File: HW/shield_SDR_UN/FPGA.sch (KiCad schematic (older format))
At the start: 68 parts, among them J1 Conn_02x09_Odd_Even, J2 Conn_02x08_Odd_Even, U4 XC6SLX9-2TQG144C, X2 ASE-xxxMHz

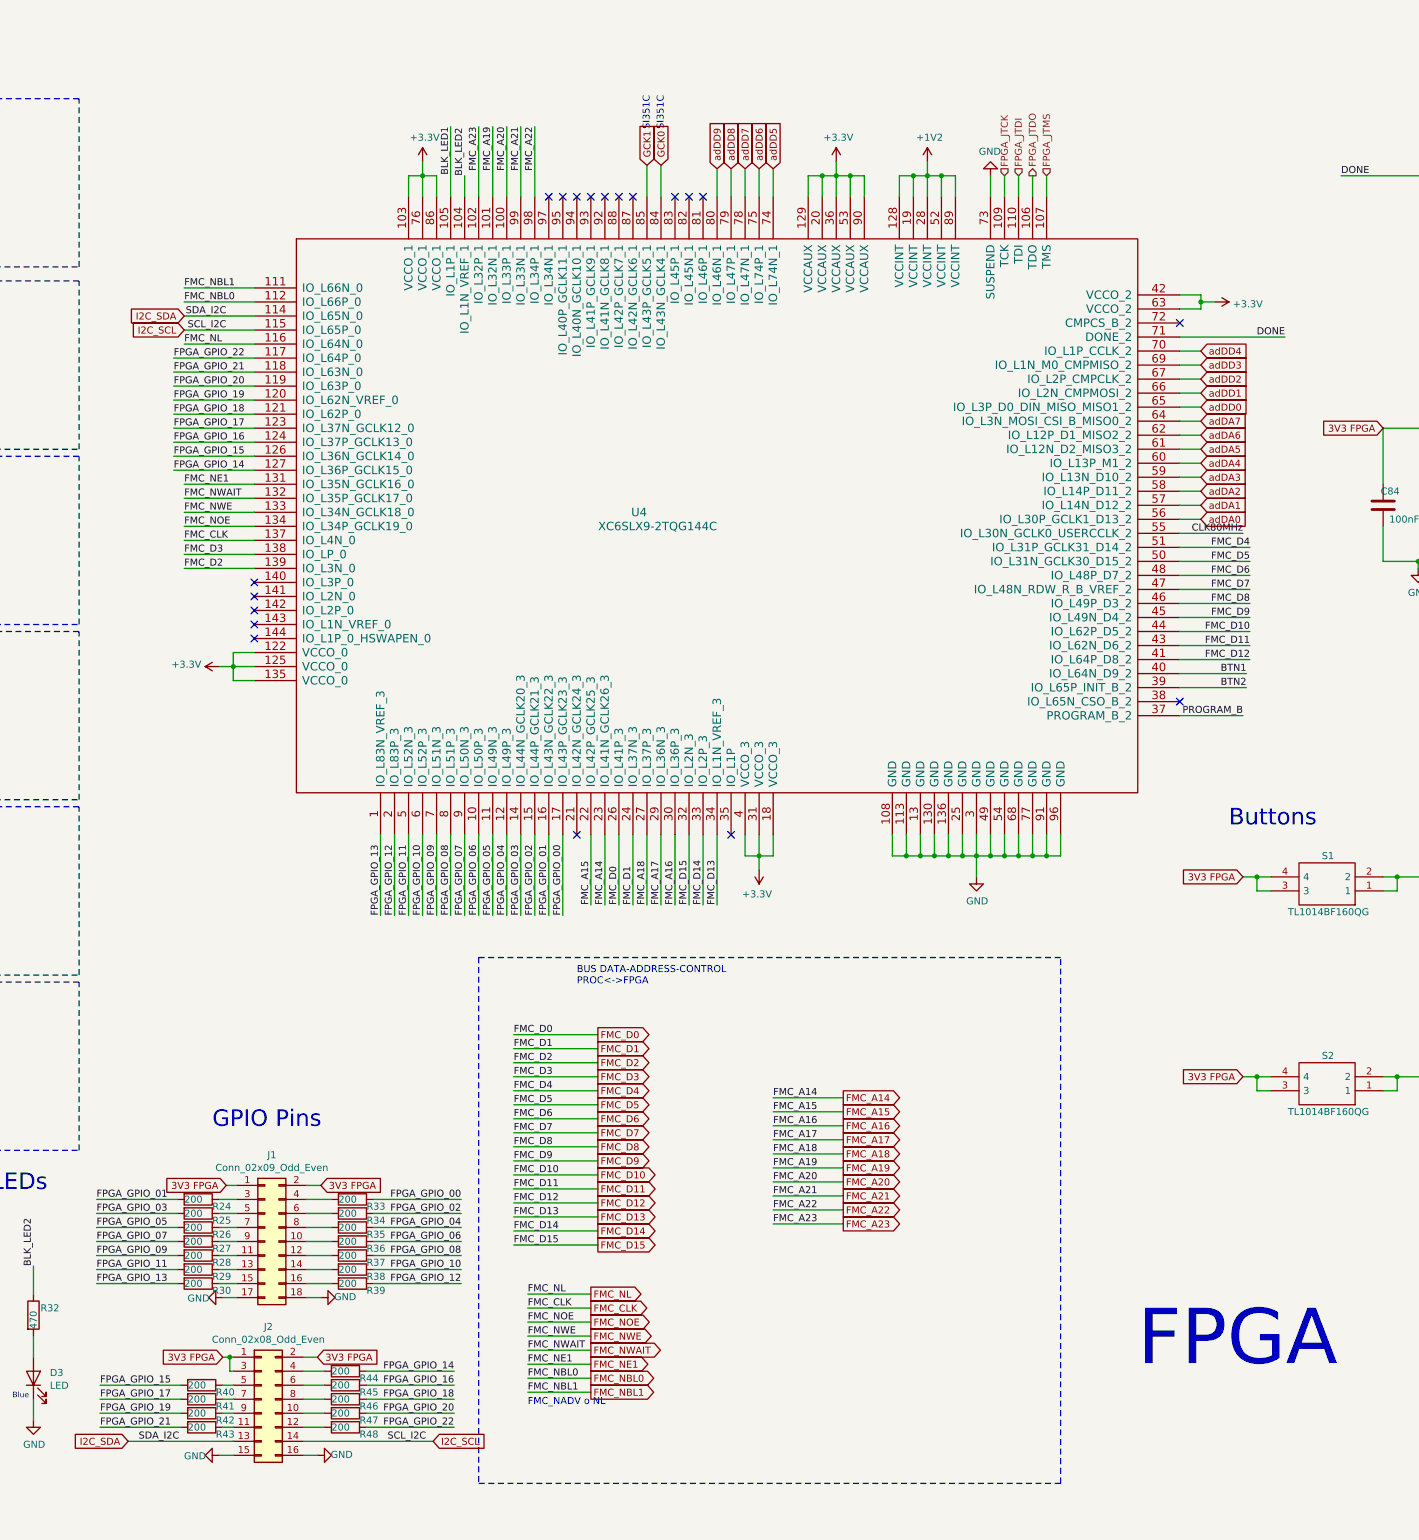
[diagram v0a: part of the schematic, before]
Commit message: PCB route V3
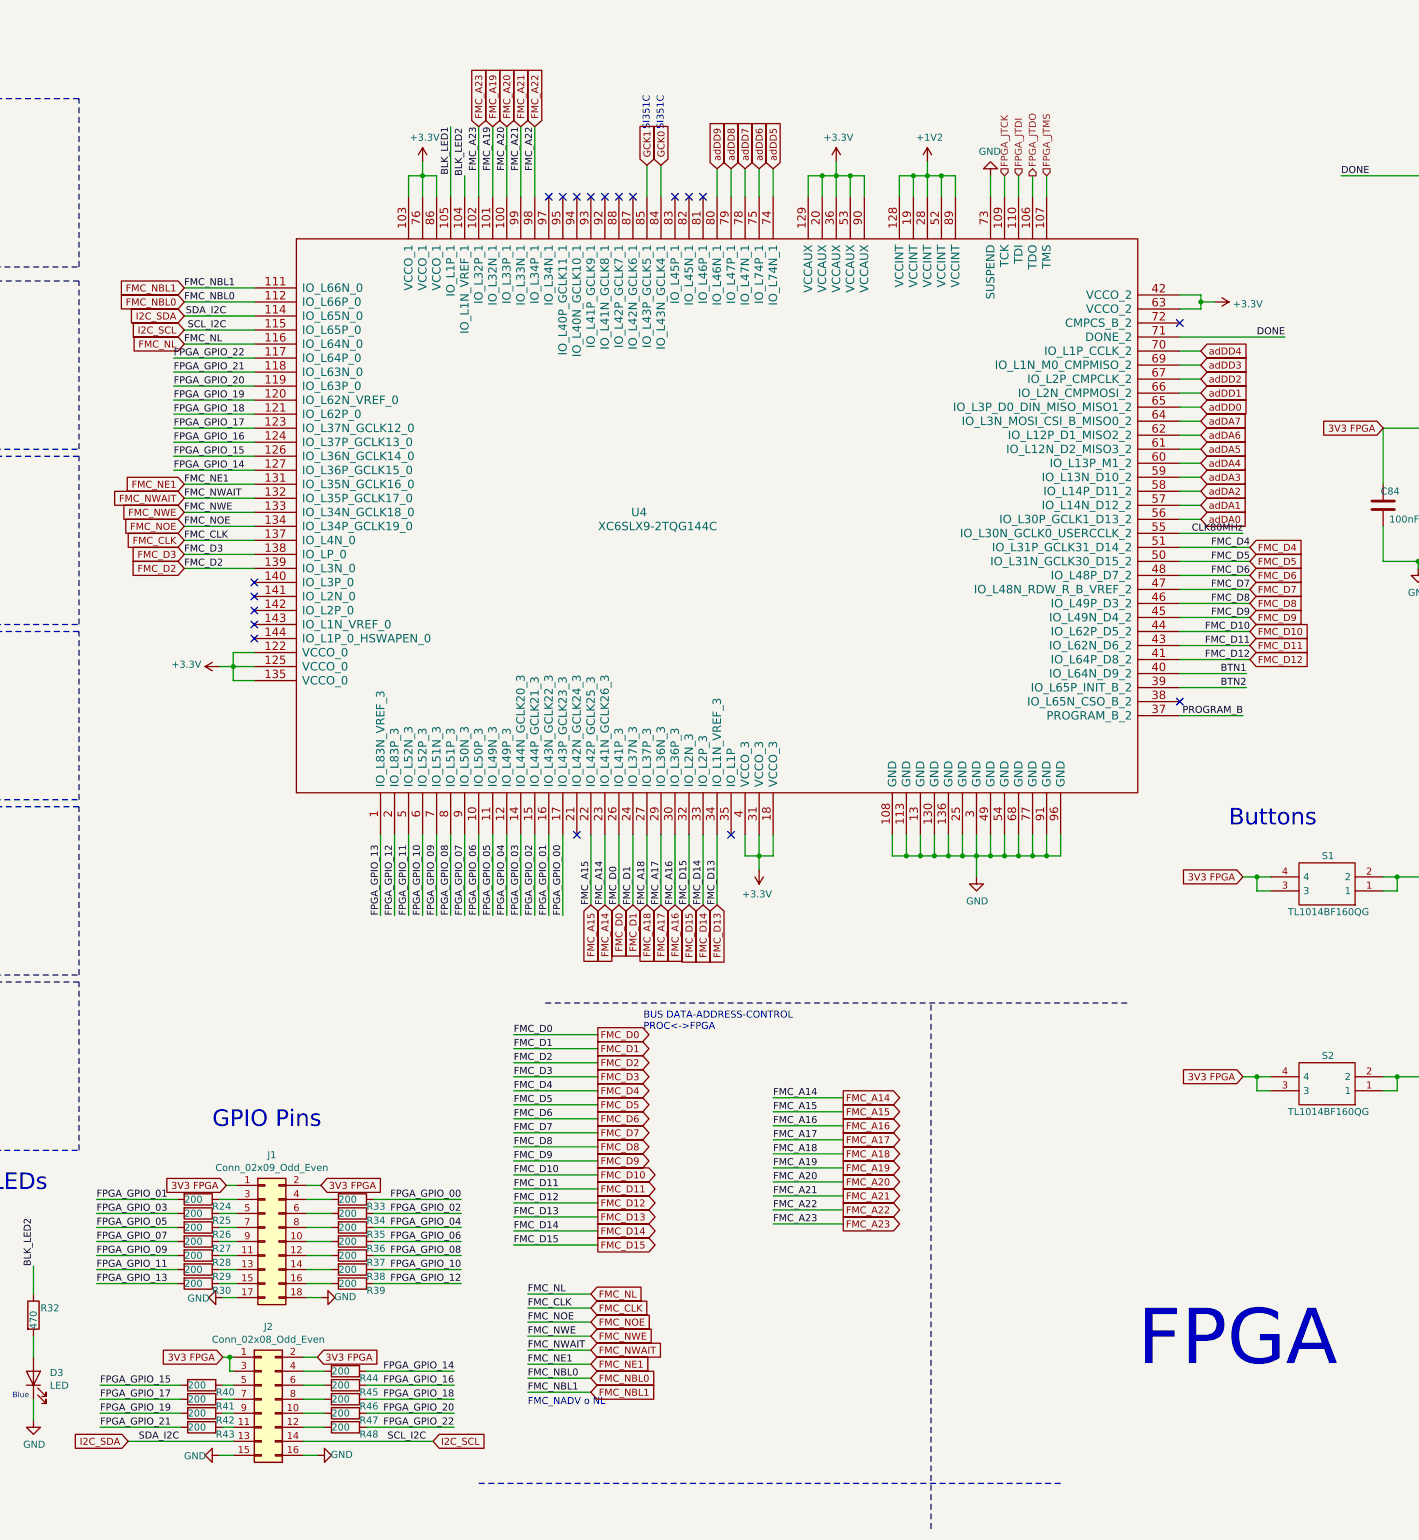
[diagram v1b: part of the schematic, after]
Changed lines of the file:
@@
 	9300 8525 9800 8525
 Wire Notes Line
-	7200 7525 7200 11275
-Wire Notes Line
-	11350 7525 7200 7525
-Text Notes 7900 7725 0    50   ~ 0
+	11825 7850 7675 7850
+Text Notes 8375 8050 0    50   ~ 0
 BUS DATA-ADDRESS-CONTROL \nPROC<->FPGA\n
 Text Label 8200 7150 1    50   ~ 0
@@
 Text Label 5100 4550 0    50   ~ 0
 FMC_CLK
-Text Label 5100 4350 0    50   ~ 0
-FMC_NWE
-Text Label 5100 4150 0    50   ~ 0
-FMC_NE1
 Text Label 5100 4450 0    50   ~ 0
 FMC_NOE
@@
 	8200 7150 8200 6650
 Wire Notes Line
-	11350 11275 11350 7525
+	10425 11600 10425 7850
 Wire Notes Line
 	7200 11275 11350 11275
@@
 Wire Wire Line
 	5100 4250 5600 4250
-Text Label 5100 4250 0    50   ~ 0
-FMC_NWAIT
 Wire Wire Line
 	8800 7150 8800 6650
@@
 Text Label 7550 10025 0    50   ~ 0
 FMC_CLK
-Text Label 7550 10225 0    50   ~ 0
-FMC_NWE
-Text Label 7550 10325 0    50   ~ 0
-FMC_NWAIT
-Text Label 7550 10425 0    50   ~ 0
-FMC_NE1
 Text Label 7550 10125 0    50   ~ 0
 FMC_NOE
@@
 Wire Wire Line
 	8000 10125 7550 10125
-Text GLabel 8000 9925 2    50   Output ~ 0
+Text GLabel 8000 9925 2    50   Input ~ 0
 FMC_NL
-Text GLabel 8000 10025 2    50   Output ~ 0
+Text GLabel 8000 10025 2    50   Input ~ 0
 FMC_CLK
-Text GLabel 8000 10125 2    50   Output ~ 0
+Text GLabel 8000 10125 2    50   Input ~ 0
 FMC_NOE
-Text GLabel 8000 10225 2    50   Output ~ 0
+Text GLabel 8000 10225 2    50   Input ~ 0
 FMC_NWE
-Text GLabel 8000 10325 2    50   Output ~ 0
+Text GLabel 8000 10325 2    50   Input ~ 0
 FMC_NWAIT
-Text GLabel 8000 10425 2    50   Output ~ 0
-FMC_NE1
-Text GLabel 8000 10525 2    50   Output ~ 0
+Text GLabel 8000 10525 2    50   Input ~ 0
 FMC_NBL0
-Text GLabel 8000 10625 2    50   Output ~ 0
+Text GLabel 8000 10625 2    50   Input ~ 0
 FMC_NBL1
 Text Label 4775 10975 0    50   ~ 0
@@
 Wire Wire Line
 	4700 10975 5450 10975
+Text Label 7550 10225 0    50   ~ 0
+FMC_NWE
+Text Label 5100 4350 0    50   ~ 0
+FMC_NWE
+Text GLabel 8000 10425 2    50   Input ~ 0
+FMC_NE1
+Text Label 5100 4250 0    50   ~ 0
+FMC_NWAIT
+Text Label 5100 4150 0    50   ~ 0
+FMC_NE1
+Text Label 7550 10425 0    50   ~ 0
+FMC_NE1
+Text Label 7550 10325 0    50   ~ 0
+FMC_NWAIT
+Text GLabel 5100 4450 0    50   Input ~ 0
+FMC_NOE
+Text GLabel 5100 4550 0    50   Input ~ 0
+FMC_CLK
+Text GLabel 5100 4350 0    50   Input ~ 0
+FMC_NWE
+Text GLabel 5100 4250 0    50   Input ~ 0
+FMC_NWAIT
+Text GLabel 5100 4150 0    50   Input ~ 0
+FMC_NE1
+Text GLabel 5100 2850 0    50   Input ~ 0
+FMC_NBL0
+Text GLabel 5100 2750 0    50   Input ~ 0
+FMC_NBL1
+Text GLabel 5100 3150 0    50   Input ~ 0
+FMC_NL
+Text GLabel 5100 4750 0    50   Input ~ 0
+FMC_D2
+Text GLabel 5100 4650 0    50   Input ~ 0
+FMC_D3
+Text GLabel 12700 4900 2    50   Input ~ 0
+FMC_D7
+Text GLabel 12700 4600 2    50   Input ~ 0
+FMC_D4
+Text GLabel 12700 4800 2    50   Input ~ 0
+FMC_D6
+Text GLabel 12700 4700 2    50   Input ~ 0
+FMC_D5
+Text GLabel 12700 5300 2    50   Input ~ 0
+FMC_D11
+Text GLabel 12700 5000 2    50   Input ~ 0
+FMC_D8
+Text GLabel 12700 5200 2    50   Input ~ 0
+FMC_D10
+Text GLabel 12700 5100 2    50   Input ~ 0
+FMC_D9
+Text GLabel 8700 7150 3    50   Input ~ 0
+FMC_D15
+Text GLabel 12700 5400 2    50   Input ~ 0
+FMC_D12
+Text GLabel 8800 7150 3    50   Input ~ 0
+FMC_D14
+Text GLabel 8900 7150 3    50   Input ~ 0
+FMC_D13
+Text GLabel 8300 7150 3    50   Input ~ 0
+FMC_D1
+Text GLabel 8200 7150 3    50   Input ~ 0
+FMC_D0
+Text GLabel 8600 7150 3    50   Input ~ 0
+FMC_A16
+Text GLabel 8500 7150 3    50   Input ~ 0
+FMC_A17
+Text GLabel 8400 7150 3    50   Input ~ 0
+FMC_A18
+Text GLabel 7300 1600 1    50   Input ~ 0
+FMC_A19
+Text GLabel 7400 1600 1    50   Input ~ 0
+FMC_A20
+Text GLabel 7500 1600 1    50   Input ~ 0
+FMC_A21
+Text GLabel 7600 1600 1    50   Input ~ 0
+FMC_A22
+Text GLabel 7200 1600 1    50   Input ~ 0
+FMC_A23
+Text GLabel 8000 7150 3    50   Input ~ 0
+FMC_A15
+Text GLabel 8100 7150 3    50   Input ~ 0
+FMC_A14
 $EndSCHEMATC
